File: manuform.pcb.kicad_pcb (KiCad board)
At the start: 2 copper layers, 90 x 90.5 mm, 55 parts, among them J1 Conn_01x05, J3 Conn_01x01, J4 Conn_01x01, SW1 SW_DIP_x01, SW2 SW_DIP_x01, SW3 SW_DIP_x01, SW4 SW_DIP_x01

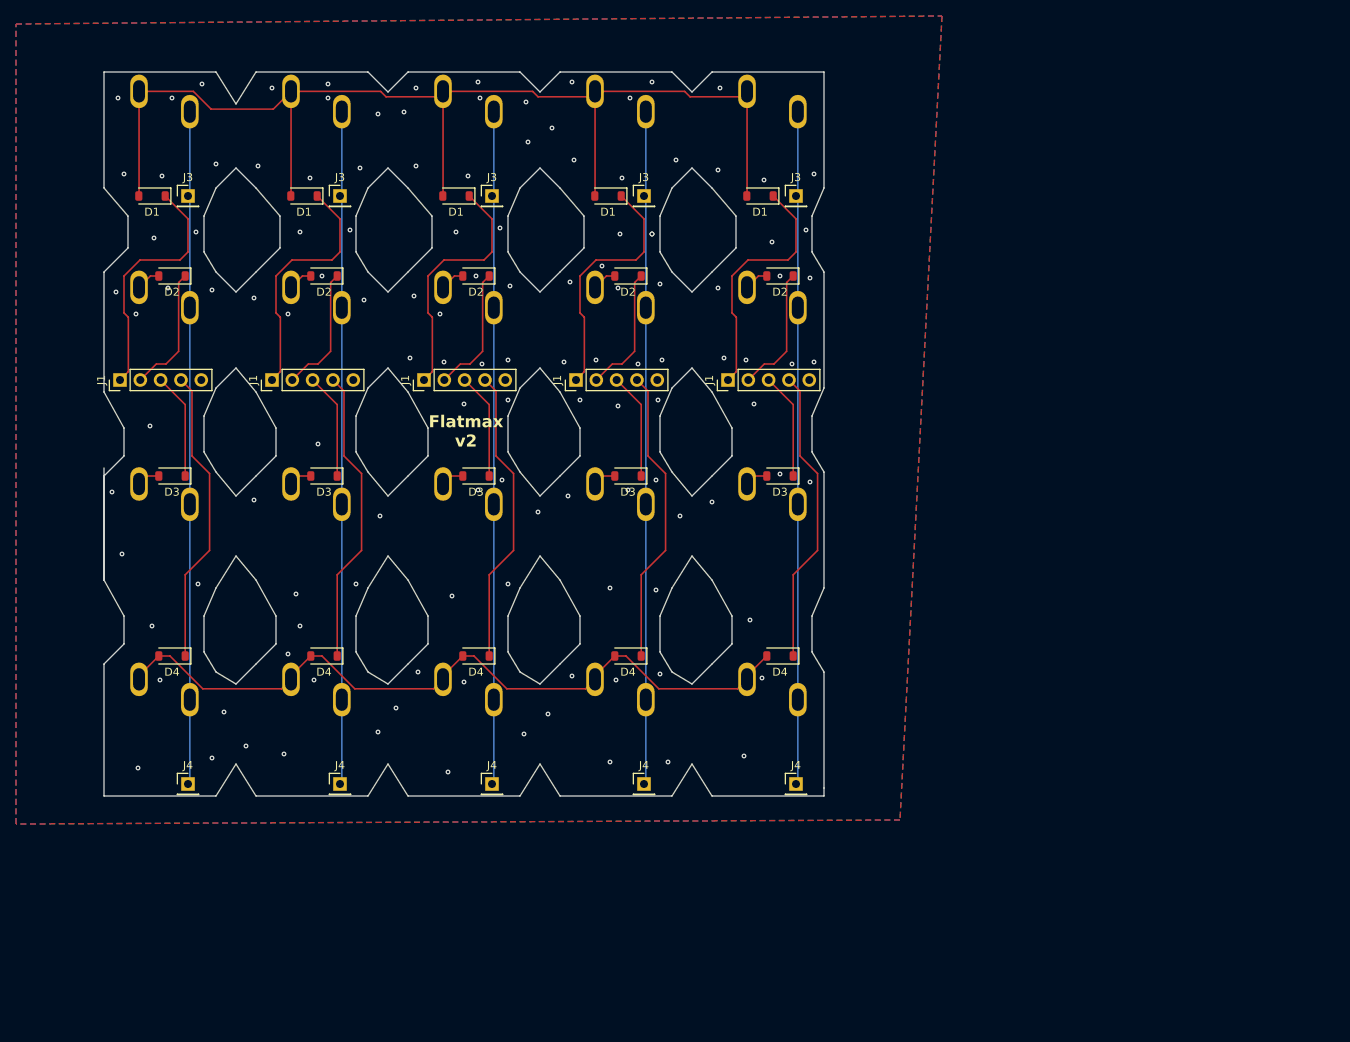
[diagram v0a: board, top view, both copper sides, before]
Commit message: 6 rows MX v1.0
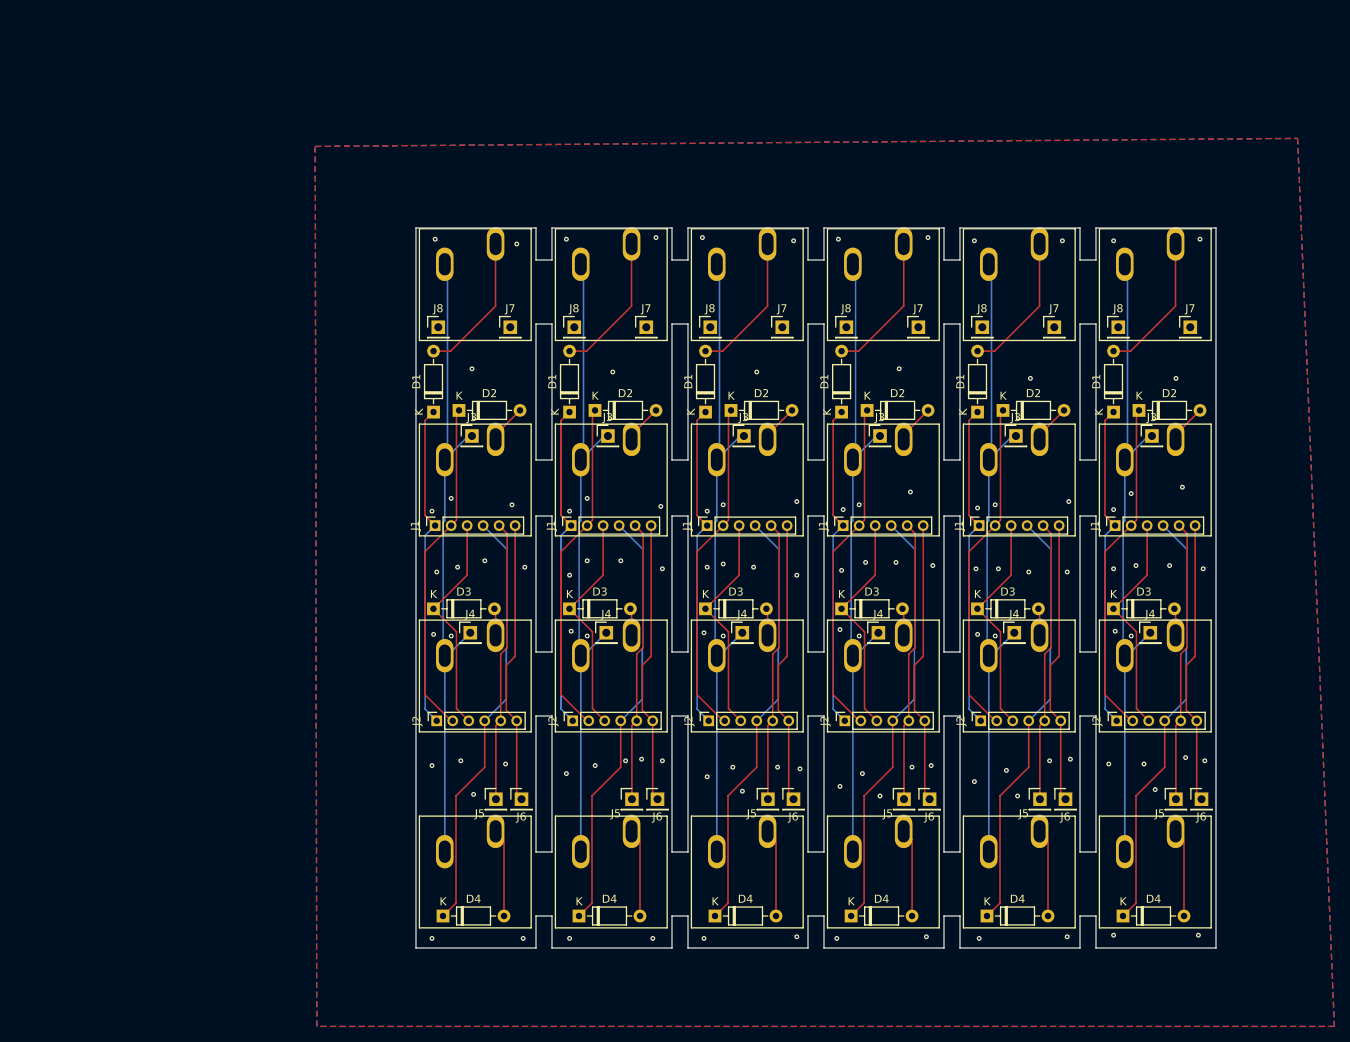
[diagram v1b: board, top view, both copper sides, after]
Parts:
- removed the D1 at (178.0, 33.0)
- removed the D1 at (121.0, 33.0)
- removed the D1 at (159.0, 33.0)
- removed the D1 at (197.0, 33.0)
- removed the D1 at (140.0, 33.0)
- removed the D2 at (199.5, 43.0)
- removed the D2 at (142.5, 43.0)
- removed the D2 at (123.5, 43.0)
- removed the D2 at (180.5, 43.0)
- removed the D2 at (161.5, 43.0)
- removed the D3 at (199.5, 68.0)
- removed the D3 at (123.5, 68.0)
- removed the D3 at (180.5, 68.0)
- removed the D3 at (142.5, 68.0)
- removed the D3 at (161.5, 68.0)
- removed the D4 at (199.5, 90.5)
- removed the D4 at (123.5, 90.5)
- removed the D4 at (180.5, 90.5)
- removed the D4 at (142.5, 90.5)
- removed the D4 at (161.5, 90.5)
- removed the J1 at (117.0, 56.0)
- removed the J1 at (193.0, 56.0)
- removed the J1 at (155.0, 56.0)
- removed the J1 at (136.0, 56.0)
- removed the J1 at (174.0, 56.0)
- removed the J3 at (125.5, 33.0)
- removed the J3 at (163.5, 33.0)
- removed the J3 at (182.5, 33.0)
- removed the J3 at (144.5, 33.0)
- removed the J3 at (201.5, 33.0)
- removed the J4 at (163.5, 106.5)
- removed the J4 at (201.5, 106.5)
- removed the J4 at (182.5, 106.5)
- removed the J4 at (144.5, 106.5)
- removed the J4 at (125.5, 106.5)
- removed the SW1 at (119.4, 19.9)
- removed the SW1 at (176.4, 19.9)
- removed the SW1 at (157.4, 19.9)
- removed the SW1 at (138.4, 19.9)
- removed the SW1 at (195.4, 19.9)
- removed the SW2 at (119.4, 44.4)
- removed the SW2 at (157.4, 44.4)
- removed the SW2 at (195.4, 44.4)
- removed the SW2 at (176.4, 44.4)
- removed the SW2 at (138.4, 44.4)
- removed the SW3 at (138.4, 69.0)
- removed the SW3 at (195.4, 69.0)
- removed the SW3 at (119.4, 69.0)
- removed the SW3 at (176.4, 69.0)
- removed the SW3 at (157.4, 69.0)
- removed the SW4 at (119.4, 93.4)
- removed the SW4 at (157.4, 93.4)
- removed the SW4 at (138.4, 93.4)
- removed the SW4 at (195.4, 93.4)
- removed the SW4 at (176.4, 93.4)
- added D1: D, Diode_THT:D_DO-35_SOD27_P7.62mm_Horizontal, F.Cu at (207.2, 60.0)
- added D1: D, Diode_THT:D_DO-35_SOD27_P7.62mm_Horizontal, F.Cu at (224.2, 60.0)
- added D1: D, Diode_THT:D_DO-35_SOD27_P7.62mm_Horizontal, F.Cu at (173.2, 60.0)
- added D1: D, Diode_THT:D_DO-35_SOD27_P7.62mm_Horizontal, F.Cu at (156.2, 60.0)
- added D1: D, Diode_THT:D_DO-35_SOD27_P7.62mm_Horizontal, F.Cu at (241.2, 60.0)
- added D1: D, Diode_THT:D_DO-35_SOD27_P7.62mm_Horizontal, F.Cu at (190.2, 60.0)
- added D2: D, Diode_THT:D_DO-35_SOD27_P7.62mm_Horizontal, F.Cu at (227.4, 59.8)
- added D2: D, Diode_THT:D_DO-35_SOD27_P7.62mm_Horizontal, F.Cu at (210.4, 59.8)
- added D2: D, Diode_THT:D_DO-35_SOD27_P7.62mm_Horizontal, F.Cu at (244.4, 59.8)
- added D2: D, Diode_THT:D_DO-35_SOD27_P7.62mm_Horizontal, F.Cu at (193.4, 59.8)
- added D2: D, Diode_THT:D_DO-35_SOD27_P7.62mm_Horizontal, F.Cu at (176.4, 59.8)
- added D2: D, Diode_THT:D_DO-35_SOD27_P7.62mm_Horizontal, F.Cu at (159.4, 59.8)
- added D3: D, Diode_THT:D_DO-35_SOD27_P7.62mm_Horizontal, F.Cu at (190.2, 84.6)
- added D3: D, Diode_THT:D_DO-35_SOD27_P7.62mm_Horizontal, F.Cu at (207.2, 84.6)
- added D3: D, Diode_THT:D_DO-35_SOD27_P7.62mm_Horizontal, F.Cu at (224.2, 84.6)
- added D3: D, Diode_THT:D_DO-35_SOD27_P7.62mm_Horizontal, F.Cu at (173.2, 84.6)
- added D3: D, Diode_THT:D_DO-35_SOD27_P7.62mm_Horizontal, F.Cu at (241.2, 84.6)
- added D3: D, Diode_THT:D_DO-35_SOD27_P7.62mm_Horizontal, F.Cu at (156.2, 84.6)
- added D4: D, Diode_THT:D_DO-35_SOD27_P7.62mm_Horizontal, F.Cu at (157.4, 123.0)
- added D4: D, Diode_THT:D_DO-35_SOD27_P7.62mm_Horizontal, F.Cu at (242.4, 123.0)
- added D4: D, Diode_THT:D_DO-35_SOD27_P7.62mm_Horizontal, F.Cu at (174.4, 123.0)
- added D4: D, Diode_THT:D_DO-35_SOD27_P7.62mm_Horizontal, F.Cu at (208.4, 123.0)
- added D4: D, Diode_THT:D_DO-35_SOD27_P7.62mm_Horizontal, F.Cu at (191.4, 123.0)
- added D4: D, Diode_THT:D_DO-35_SOD27_P7.62mm_Horizontal, F.Cu at (225.4, 123.0)
- added J1: Conn_01x06, Connector_PinSocket_2.00mm:PinSocket_1x06_P2.00mm_Vertical, F.Cu at (156.4, 74.2)
- added J1: Conn_01x06, Connector_PinSocket_2.00mm:PinSocket_1x06_P2.00mm_Vertical, F.Cu at (241.4, 74.2)
- added J1: Conn_01x06, Connector_PinSocket_2.00mm:PinSocket_1x06_P2.00mm_Vertical, F.Cu at (190.4, 74.2)
- added J1: Conn_01x06, Connector_PinSocket_2.00mm:PinSocket_1x06_P2.00mm_Vertical, F.Cu at (224.4, 74.2)
- added J1: Conn_01x06, Connector_PinSocket_2.00mm:PinSocket_1x06_P2.00mm_Vertical, F.Cu at (207.4, 74.2)
- added J1: Conn_01x06, Connector_PinSocket_2.00mm:PinSocket_1x06_P2.00mm_Vertical, F.Cu at (173.4, 74.2)
- added J2: Conn_01x06, Connector_PinSocket_2.00mm:PinSocket_1x06_P2.00mm_Vertical, F.Cu at (190.6, 98.6)
- added J2: Conn_01x06, Connector_PinSocket_2.00mm:PinSocket_1x06_P2.00mm_Vertical, F.Cu at (207.6, 98.6)
- added J2: Conn_01x06, Connector_PinSocket_2.00mm:PinSocket_1x06_P2.00mm_Vertical, F.Cu at (173.6, 98.6)
- added J2: Conn_01x06, Connector_PinSocket_2.00mm:PinSocket_1x06_P2.00mm_Vertical, F.Cu at (224.6, 98.6)
- added J2: Conn_01x06, Connector_PinSocket_2.00mm:PinSocket_1x06_P2.00mm_Vertical, F.Cu at (156.6, 98.6)
- added J2: Conn_01x06, Connector_PinSocket_2.00mm:PinSocket_1x06_P2.00mm_Vertical, F.Cu at (241.6, 98.6)
- added J3: Conn_01x01, Connector_PinHeader_2.54mm:PinHeader_1x01_P2.54mm_Vertical, F.Cu at (229.0, 63.0)
- added J3: Conn_01x01, Connector_PinHeader_2.54mm:PinHeader_1x01_P2.54mm_Vertical, F.Cu at (178.0, 63.0)
- added J3: Conn_01x01, Connector_PinHeader_2.54mm:PinHeader_1x01_P2.54mm_Vertical, F.Cu at (195.0, 63.0)
- added J3: Conn_01x01, Connector_PinHeader_2.54mm:PinHeader_1x01_P2.54mm_Vertical, F.Cu at (161.0, 63.0)
- added J3: Conn_01x01, Connector_PinHeader_2.54mm:PinHeader_1x01_P2.54mm_Vertical, F.Cu at (212.0, 63.0)
- added J3: Conn_01x01, Connector_PinHeader_2.54mm:PinHeader_1x01_P2.54mm_Vertical, F.Cu at (246.0, 63.0)
- added J4: Conn_01x01, Connector_PinHeader_2.54mm:PinHeader_1x01_P2.54mm_Vertical, F.Cu at (177.8, 87.6)
- added J4: Conn_01x01, Connector_PinHeader_2.54mm:PinHeader_1x01_P2.54mm_Vertical, F.Cu at (160.8, 87.6)
- added J4: Conn_01x01, Connector_PinHeader_2.54mm:PinHeader_1x01_P2.54mm_Vertical, F.Cu at (245.8, 87.6)
- added J4: Conn_01x01, Connector_PinHeader_2.54mm:PinHeader_1x01_P2.54mm_Vertical, F.Cu at (228.8, 87.6)
- added J4: Conn_01x01, Connector_PinHeader_2.54mm:PinHeader_1x01_P2.54mm_Vertical, F.Cu at (194.8, 87.6)
- added J4: Conn_01x01, Connector_PinHeader_2.54mm:PinHeader_1x01_P2.54mm_Vertical, F.Cu at (211.8, 87.6)
- added J5: Conn_01x01, Connector_PinHeader_2.54mm:PinHeader_1x01_P2.54mm_Vertical, F.Cu at (164.0, 108.4)
- added J5: Conn_01x01, Connector_PinHeader_2.54mm:PinHeader_1x01_P2.54mm_Vertical, F.Cu at (181.0, 108.4)
- added J5: Conn_01x01, Connector_PinHeader_2.54mm:PinHeader_1x01_P2.54mm_Vertical, F.Cu at (232.0, 108.4)
- added J5: Conn_01x01, Connector_PinHeader_2.54mm:PinHeader_1x01_P2.54mm_Vertical, F.Cu at (198.0, 108.4)
- added J5: Conn_01x01, Connector_PinHeader_2.54mm:PinHeader_1x01_P2.54mm_Vertical, F.Cu at (249.0, 108.4)
- added J5: Conn_01x01, Connector_PinHeader_2.54mm:PinHeader_1x01_P2.54mm_Vertical, F.Cu at (215.0, 108.4)
- added J6: Conn_01x01, Connector_PinHeader_2.54mm:PinHeader_1x01_P2.54mm_Vertical, F.Cu at (167.2, 108.4)
- added J6: Conn_01x01, Connector_PinHeader_2.54mm:PinHeader_1x01_P2.54mm_Vertical, F.Cu at (218.2, 108.4)
- added J6: Conn_01x01, Connector_PinHeader_2.54mm:PinHeader_1x01_P2.54mm_Vertical, F.Cu at (201.2, 108.4)
- added J6: Conn_01x01, Connector_PinHeader_2.54mm:PinHeader_1x01_P2.54mm_Vertical, F.Cu at (235.2, 108.4)
- added J6: Conn_01x01, Connector_PinHeader_2.54mm:PinHeader_1x01_P2.54mm_Vertical, F.Cu at (252.2, 108.4)
- added J6: Conn_01x01, Connector_PinHeader_2.54mm:PinHeader_1x01_P2.54mm_Vertical, F.Cu at (184.2, 108.4)
- added J7: Conn_01x01, Connector_PinHeader_2.54mm:PinHeader_1x01_P2.54mm_Vertical, F.Cu at (182.8, 49.4)
- added J7: Conn_01x01, Connector_PinHeader_2.54mm:PinHeader_1x01_P2.54mm_Vertical, F.Cu at (250.8, 49.4)
- added J7: Conn_01x01, Connector_PinHeader_2.54mm:PinHeader_1x01_P2.54mm_Vertical, F.Cu at (216.8, 49.4)
- added J7: Conn_01x01, Connector_PinHeader_2.54mm:PinHeader_1x01_P2.54mm_Vertical, F.Cu at (165.8, 49.4)
- added J7: Conn_01x01, Connector_PinHeader_2.54mm:PinHeader_1x01_P2.54mm_Vertical, F.Cu at (233.8, 49.4)
- added J7: Conn_01x01, Connector_PinHeader_2.54mm:PinHeader_1x01_P2.54mm_Vertical, F.Cu at (199.8, 49.4)
- added J8: Conn_01x01, Connector_PinHeader_2.54mm:PinHeader_1x01_P2.54mm_Vertical, F.Cu at (241.8, 49.4)
- added J8: Conn_01x01, Connector_PinHeader_2.54mm:PinHeader_1x01_P2.54mm_Vertical, F.Cu at (190.8, 49.4)
- added J8: Conn_01x01, Connector_PinHeader_2.54mm:PinHeader_1x01_P2.54mm_Vertical, F.Cu at (173.8, 49.4)
- added J8: Conn_01x01, Connector_PinHeader_2.54mm:PinHeader_1x01_P2.54mm_Vertical, F.Cu at (224.8, 49.4)
- added J8: Conn_01x01, Connector_PinHeader_2.54mm:PinHeader_1x01_P2.54mm_Vertical, F.Cu at (207.8, 49.4)
- added J8: Conn_01x01, Connector_PinHeader_2.54mm:PinHeader_1x01_P2.54mm_Vertical, F.Cu at (156.8, 49.4)
- added SW1: SW_DIP_x01, switchCustom:SW_Cherry_MX_1.00u_PCB, F.Cu at (248.9, 39.0)
- added SW1: SW_DIP_x01, switchCustom:SW_Cherry_MX_1.00u_PCB, F.Cu at (180.9, 39.0)
- added SW1: SW_DIP_x01, switchCustom:SW_Cherry_MX_1.00u_PCB, F.Cu at (231.9, 39.0)
- added SW1: SW_DIP_x01, switchCustom:SW_Cherry_MX_1.00u_PCB, F.Cu at (197.9, 39.0)
- added SW1: SW_DIP_x01, switchCustom:SW_Cherry_MX_1.00u_PCB, F.Cu at (163.9, 39.0)
- added SW1: SW_DIP_x01, switchCustom:SW_Cherry_MX_1.00u_PCB, F.Cu at (215.0, 39.0)
- added SW2: SW_DIP_x01, switchCustom:SW_Cherry_MX_1.00u_PCB, F.Cu at (197.9, 63.4)
- added SW2: SW_DIP_x01, switchCustom:SW_Cherry_MX_1.00u_PCB, F.Cu at (231.9, 63.4)
- added SW2: SW_DIP_x01, switchCustom:SW_Cherry_MX_1.00u_PCB, F.Cu at (215.0, 63.4)
- added SW2: SW_DIP_x01, switchCustom:SW_Cherry_MX_1.00u_PCB, F.Cu at (248.9, 63.4)
- added SW2: SW_DIP_x01, switchCustom:SW_Cherry_MX_1.00u_PCB, F.Cu at (180.9, 63.4)
- added SW2: SW_DIP_x01, switchCustom:SW_Cherry_MX_1.00u_PCB, F.Cu at (163.9, 63.4)
- added SW3: SW_DIP_x01, switchCustom:SW_Cherry_MX_1.00u_PCB, F.Cu at (248.9, 87.9)
- added SW3: SW_DIP_x01, switchCustom:SW_Cherry_MX_1.00u_PCB, F.Cu at (180.9, 87.9)
- added SW3: SW_DIP_x01, switchCustom:SW_Cherry_MX_1.00u_PCB, F.Cu at (215.0, 87.9)
- added SW3: SW_DIP_x01, switchCustom:SW_Cherry_MX_1.00u_PCB, F.Cu at (197.9, 87.9)
- added SW3: SW_DIP_x01, switchCustom:SW_Cherry_MX_1.00u_PCB, F.Cu at (163.9, 87.9)
- added SW3: SW_DIP_x01, switchCustom:SW_Cherry_MX_1.00u_PCB, F.Cu at (231.9, 87.9)
- added SW4: SW_DIP_x01, switchCustom:SW_Cherry_MX_1.00u_PCB, F.Cu at (231.9, 112.4)
- added SW4: SW_DIP_x01, switchCustom:SW_Cherry_MX_1.00u_PCB, F.Cu at (248.9, 112.4)
- added SW4: SW_DIP_x01, switchCustom:SW_Cherry_MX_1.00u_PCB, F.Cu at (163.9, 112.4)
- added SW4: SW_DIP_x01, switchCustom:SW_Cherry_MX_1.00u_PCB, F.Cu at (197.9, 112.4)
- added SW4: SW_DIP_x01, switchCustom:SW_Cherry_MX_1.00u_PCB, F.Cu at (215.0, 112.4)
- added SW4: SW_DIP_x01, switchCustom:SW_Cherry_MX_1.00u_PCB, F.Cu at (180.9, 112.4)
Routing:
- net Net-(J1-Pin_6): track 0.00 -> 212.7 mm
- net Net-(J1-Pin_5): track 0.00 -> 211.2 mm
- net Net-(D2-K): track 80.1 -> 270.5 mm
- net Net-(D4-K): track 186.2 -> 320.0 mm
- net Net-(D1-K): track 155.4 -> 277.6 mm
- net Net-(D3-K): track 66.4 -> 167.8 mm
- net Net-(J3-Pin_1): track 420.7 -> 497.2 mm
- net Net-(D1-A): track 145.0 -> 107.1 mm
- net Net-(D4-A): track 94.6 -> 69.4 mm
- net Net-(D2-A): track 15.3 -> 29.3 mm
- net Net-(D3-A): track 14.4 -> 20.3 mm
- net GND: vias 128 -> 113
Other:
- board size 90 x 90.5 mm -> 100 x 90 mm
- board text added: "C"
- board text added: "Flatmax v1.0"
- board text added: "GND"
- board text added: "MX switches"
- board text added: "R5"
- board text added: "R6"
- board text removed: "Flatmax v2"
